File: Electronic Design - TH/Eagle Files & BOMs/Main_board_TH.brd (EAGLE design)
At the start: 86.2 x 145.6 mm, 37 parts, among them M1 ARDUINO-NANO-3.0, Q1 IRF9520, Q2 IRF9520

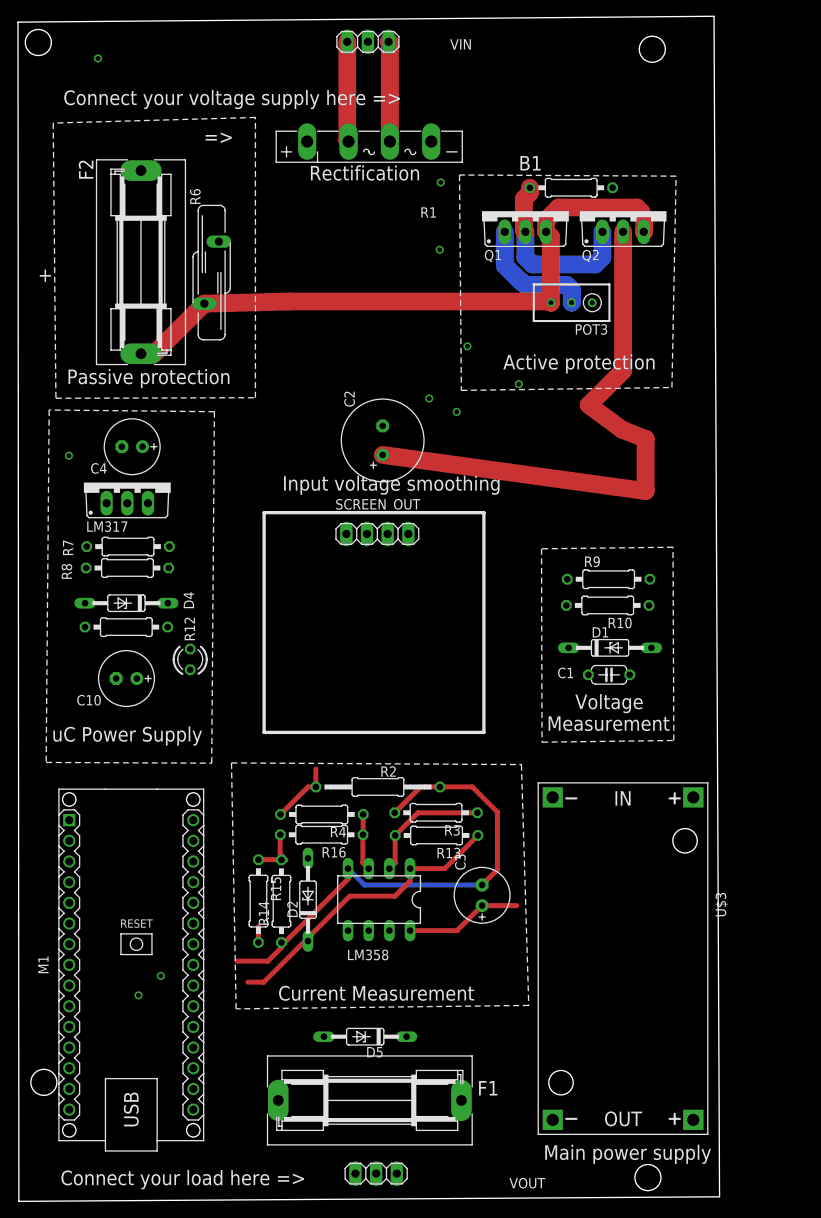
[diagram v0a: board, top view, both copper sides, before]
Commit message: high level layout complete and adding in BOM
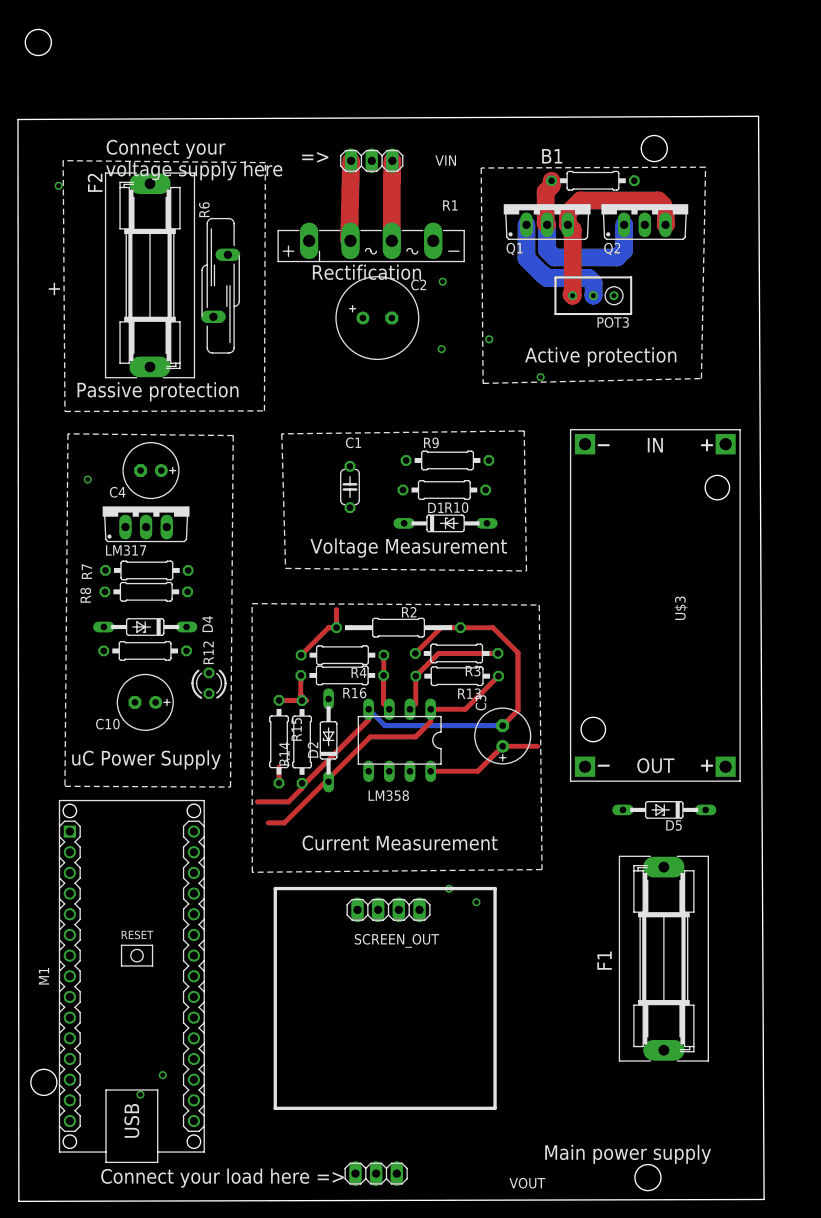
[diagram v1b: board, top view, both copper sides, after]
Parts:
- moved SCREEN_OUT 46.2 mm to (45.7, 35.3)
- moved D5 46.1 mm to (79.6, 47.5)
- moved U$3 43.6 mm to (78.5, 72.7)
- moved F1 40.1 mm to (79.6, 29.3), turned to 270 degrees
- moved C1 39.3 mm to (41.0, 87.2), turned to 90 degrees
- moved D1 25.3 mm to (52.7, 82.8)
- moved R9 24.6 mm to (53.0, 90.5)
- moved R10 24.6 mm to (52.6, 86.8)
- moved C3 19.7 mm to (59.8, 56.6)
- moved D2 19.7 mm to (38.4, 56.1)
- moved LM358 19.7 mm to (47.1, 56.1)
- moved R13 19.7 mm to (54.2, 64.0)
- moved R14 19.7 mm to (35.1, 55.9)
- moved R15 19.7 mm to (32.3, 55.9)
- moved R2 19.7 mm to (47.0, 69.9)
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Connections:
- removed net A6: M1.J2.6
- removed net A7: M1.J2.5
- removed net IIN: D2.C, LM358.1, M1.J2.12, R13.1
- new net A0: D2.C, M1.J2.12
- new net A1: M1.J2.11
- new net I_IN: LM358.1, M1.J2.6, R13.1
- new net V_IN: C1.1, D1.C, M1.J2.5, R10.2, R9.1
- net VIN: no longer C1.1, D1.C, M1.J2.11, R10.2, R9.1
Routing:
- net VIN_PROTECTED: track 84.6 -> 14.4 mm
- net VIN_UNPROTECTED: track 78.5 -> 25.8 mm
- net IIN: track 37.0 -> 0.00 mm
- net I_IN: track 0.00 -> 36.6 mm
- net N$9: track 12.3 -> 9.83 mm
- net N$7: track 12.3 -> 9.90 mm
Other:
- board size 86.2 x 145.6 mm -> 91.7 x 133.3 mm
- board text added: "Connect your voltage supply here"
- board text removed: "Connect your voltage supply here =>"
- board text removed: "Input voltage smoothing"

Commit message: completing passive protection and active protection alignment and renaming components sequentially (i.e. R1, R2, R3, ...)
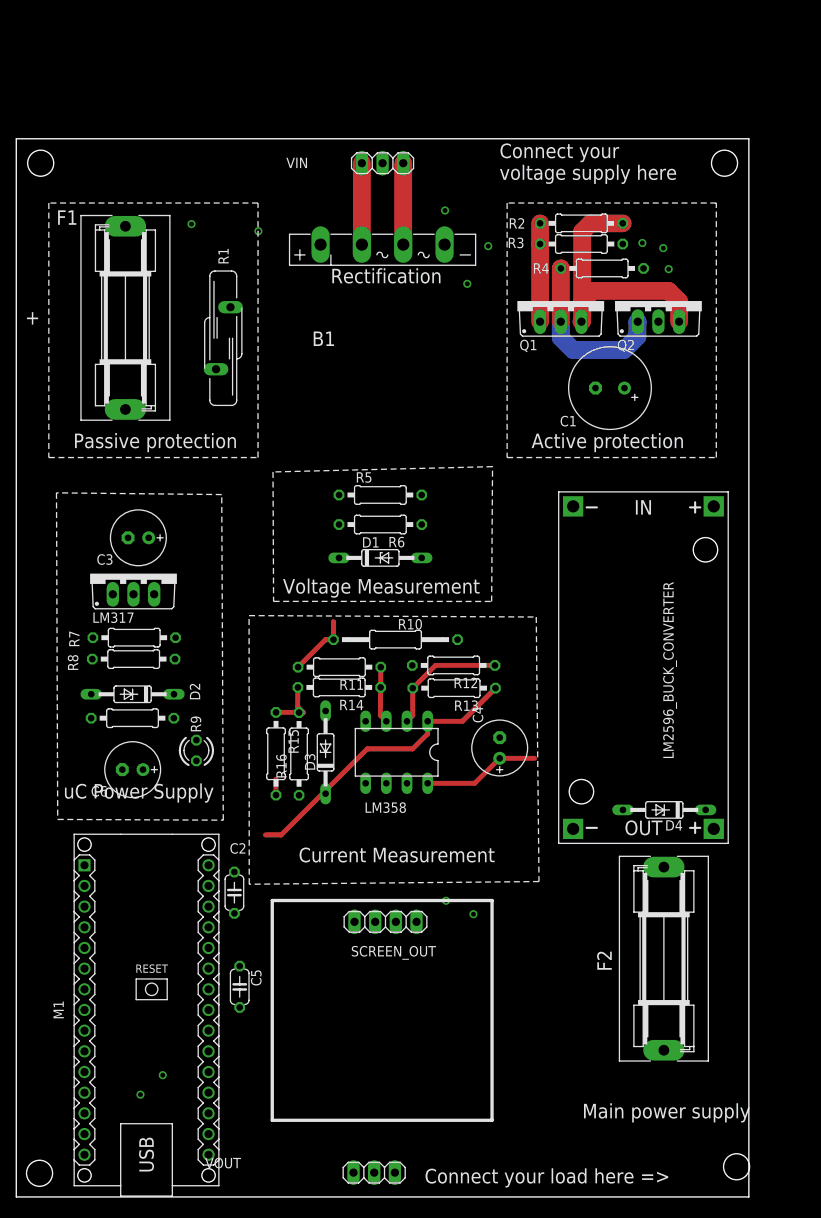
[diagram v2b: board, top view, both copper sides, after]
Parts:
- removed C10: 10u, resistor:E2,5-7
- removed D5: 5.1V, diode:DO35Z10
- removed POT3: 100k, resistor:RTRIM3296W
- removed U$3: DC-DC-STEP-DOWN-LM2596, diy-modules:DC-DC-STEP-DOWN-LM2596
- added C5: 10n, resistor:C050-024X044
- added C6: 10u, resistor:E2,5-7
- added D3: 5.1V, diode:DO35Z10
- added LM2596_BUCK_CONVERTER: DC-DC-STEP-DOWN-LM2596, diy-modules:DC-DC-STEP-DOWN-LM2596
- added R11: 1k, resistor:0207/10
- added R5: 10k, resistor:0207/10
- C1: value 10n -> 220uF; device resistor:C050-024X044 -> resistor:E3,5-10
- C2: value 220uF -> 10n; device resistor:E3,5-10 -> resistor:C050-024X044
- R1: value 100k -> S14K75; device resistor:0207/10 -> varistor:S14K17
- R10: value 1k -> 0R01; device resistor:0207/10 -> resistor:0207/15
- R12: value 2k -> 1k
- R14: value 10k -> 47k
- R16: value 47k -> 10k
- R2: value 0R01 -> 10k; device resistor:0207/15 -> resistor:0207/10
- R3: value 1k -> 10k
- R4: value 1k -> 100k
- R6: value S14K75 -> 1k; device varistor:S14K17 -> resistor:0207/10
- R9: value 10k -> 2k
- moved F2 105.0 mm to (79.6, 29.3)
- moved F1 102.8 mm to (13.4, 108.0)
- moved C2 72.7 mm to (26.8, 37.4), turned to 90 degrees
- moved D4 67.6 mm to (79.6, 47.5)
- moved R4 57.2 mm to (72.0, 114.1)
- moved C4 54.7 mm to (59.4, 55.2), turned to 90 degrees
- moved R2 54.5 mm to (69.4, 119.6), turned to 0 degrees
- moved R3 52.6 mm to (69.4, 117.1)
- moved C3 51.0 mm to (15.0, 81.0), turned to 180 degrees
- moved R9 50.0 mm to (14.3, 58.8)
- moved R1 49.4 mm to (25.4, 105.5), turned to 0 degrees
- moved R12 37.9 mm to (53.7, 65.3), turned to 180 degrees
- moved R6 35.3 mm to (44.7, 82.6), turned to 180 degrees
- moved C1 34.2 mm to (72.9, 99.4), turned to 180 degrees
- moved D2 24.7 mm to (14.3, 61.8), turned to 180 degrees
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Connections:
- removed net Q1_GATE: POT3.2, Q1.1
- new net N$3: Q1.1, R2.1, R3.2
- net +5V: now also C6.+, D2.C, R9.2; no longer C10.+, D4.C, R12.2
- net A0: no longer D2.C
- net GND: now also C1.-, C2.2, C5.2, C6.-, D3.A, R1.2, R12.2, R16.1, R3.1, R4.1, R6.1; no longer C1.2, C10.-, C2.-, D4.A, POT3.1, R1.1, R14.1, R2.1, R3.2, R6.2
- net I_IN: now also C5.1, D3.C
- net N$1: now also F1.1; no longer F2.1
- net N$10: now also D4.A, LM2596_BUCK_CONVERTER.OUT-; no longer D5.A, U$3.OUT-
- net N$2: now also R9.1; no longer R12.1
- net N$4: now also LM2596_BUCK_CONVERTER.IN-, R10.2, R11.2; no longer R2.2, R4.2, U$3.IN-
- net N$5: now also R11.1, R14.1; no longer R16.1, R4.1
- net N$6: now also R12.1; no longer R3.1
- net Q2_GATE: now also R4.2; no longer R1.2
- net VIN_PROTECTED: now also C1.+, LM2596_BUCK_CONVERTER.IN+, R5.2; no longer C2.+, R9.2, U$3.IN+
- net VIN_UNPROTECTED: now also F1.2, R1.1, R2.2; no longer F2.2, POT3.3, R6.1
- net VOUT_FINAL: now also D4.C, F2.2; no longer D5.C, F1.2
- net VOUT_PREFUSE: now also F2.1, LM2596_BUCK_CONVERTER.OUT+; no longer F1.1, U$3.OUT+
- net V_IN: now also C2.1, R5.1, R6.2; no longer C1.1, R10.2, R9.1
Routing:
- net GND: track 61.9 -> 0.00 mm, vias 10 -> 12
- net Q1_GATE: track 15.2 -> 0.00 mm
- net N$3: track 0.00 -> 12.1 mm
- net VIN_UNPROTECTED: track 25.8 -> 32.0 mm
- net Q2_GATE: track 22.2 -> 21.1 mm
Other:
- board size 91.7 x 133.3 mm -> 90 x 130 mm
